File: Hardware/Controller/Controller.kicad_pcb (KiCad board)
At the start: 2 copper layers, 40 parts, among them J2 TagConnect_SWD, Q1 Q_NMOS_GSD, Q3 Q_Dual_NMOS_S1G1S2G2D2D2D1D1, SW1 SW_Push, U1 W25Q64JVXGIQ, U2 AMS1117-3.3, U3 RP2040, U5 LTC4020, Y1 Crystal

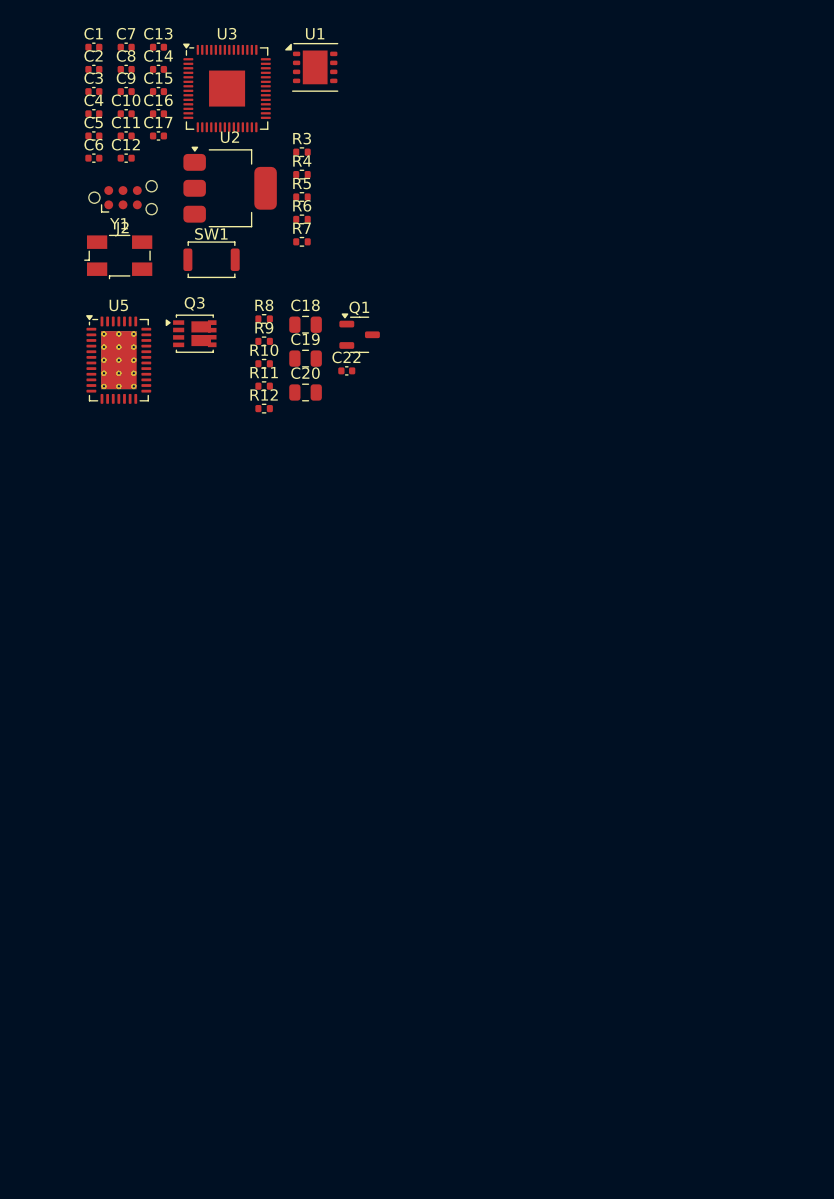
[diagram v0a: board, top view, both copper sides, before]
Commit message: User interface and Controller done
yes
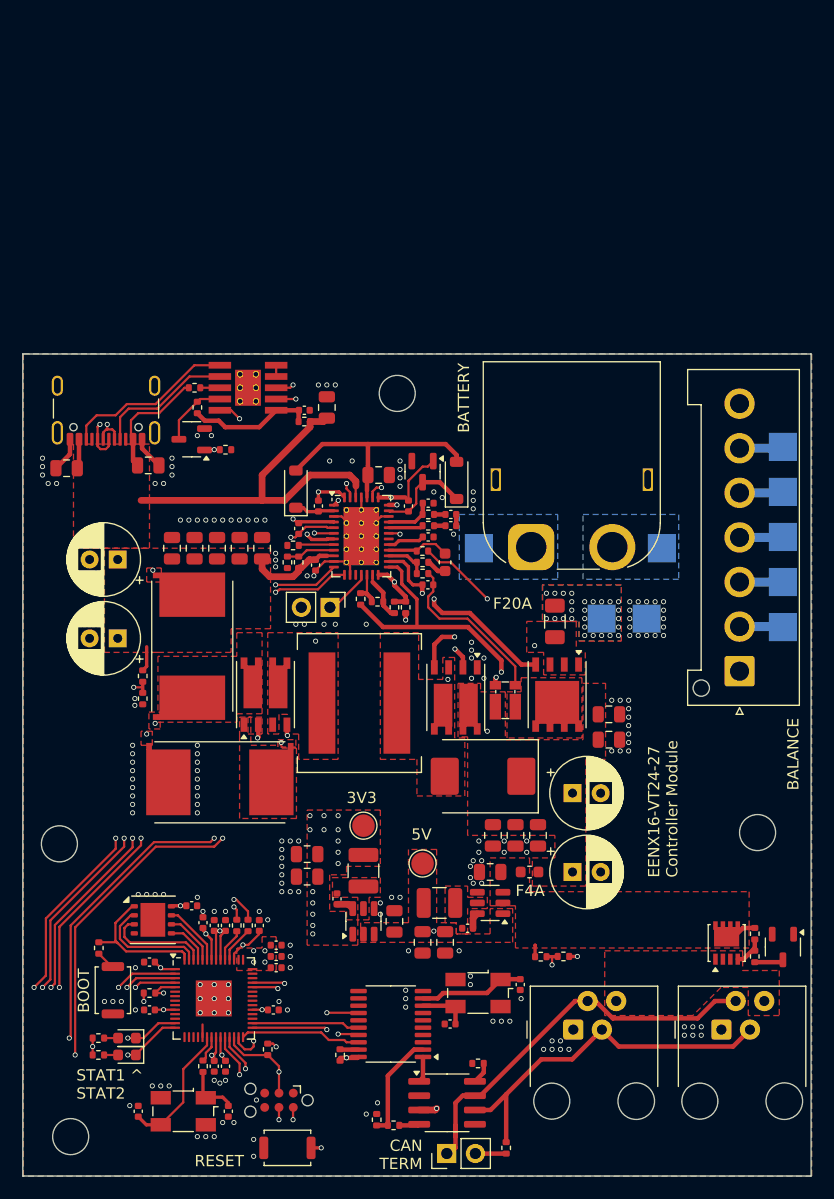
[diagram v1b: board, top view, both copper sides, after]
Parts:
- removed C1, C22, C3, C6: 1u, Capacitor_SMD:C_0402_1005Metric
- removed C10, C11, C12, C13, C14, C15, C16, C17, C2, C7, C8, C9: 100n, Capacitor_SMD:C_0402_1005Metric
- removed C18, C19, C20: 10u, Capacitor_SMD:C_0805_2012Metric
- removed C4, C5: 10p, Capacitor_SMD:C_0402_1005Metric
- removed J2: TagConnect_SWD, Connector:Tag-Connect_TC2030-IDC-NL_2x03_P1.27mm_Vertical
- removed Q1: Q_NMOS_GSD, Package_TO_SOT_SMD:SOT-23-3
- removed Q3: Q_Dual_NMOS_S1G1S2G2D2D2D1D1, Package_SO:Vishay_PowerPAK_1212-8_Dual
- removed R10, R11, R12, R6, R9: 10k, Resistor_SMD:R_0402_1005Metric
- removed R3, R7, R8: 1k, Resistor_SMD:R_0402_1005Metric
- removed R4, R5: 27, Resistor_SMD:R_0402_1005Metric
- removed SW1: SW_Push, Button_Switch_SMD:SW_Push_SPST_NO_Alps_SKRK
- removed U1: W25Q64JVXGIQ, Package_SON:WSON-8-1EP_4x4mm_P0.8mm_EP2.2x3mm
- removed U2: AMS1117-3.3, Package_TO_SOT_SMD:SOT-223-3_TabPin2
- removed U3: RP2040, Package_DFN_QFN:QFN-56-1EP_7x7mm_P0.4mm_EP3.2x3.2mm
- removed U5: LTC4020, Package_DFN_QFN:QFN-38-1EP_5x7mm_P0.5mm_EP3.15x5.15mm_ThermalVias
- removed Y1: Crystal, Crystal:Crystal_SMD_Abracon_ABM3B-4Pin_5.0x3.2mm
- added C201: 100n, Capacitor_SMD:C_0402_1005Metric, F.Cu at (117.0, 129.8)
- added C202: 100n, Capacitor_SMD:C_0402_1005Metric, F.Cu at (117.2, 126.0)
- added C203: 100n, Capacitor_SMD:C_0402_1005Metric, F.Cu at (117.2, 124.0)
- added C204: 100n, Capacitor_SMD:C_0402_1005Metric, F.Cu at (117.2, 125.0)
- added C205: 100n, Capacitor_SMD:C_0402_1005Metric, F.Cu at (112.8, 122.2)
- added C206: 100n, Capacitor_SMD:C_0402_1005Metric, F.Cu at (111.8, 122.2)
- added C207: 100n, Capacitor_SMD:C_0402_1005Metric, F.Cu at (106.0, 125.5)
- added C208: 100n, Capacitor_SMD:C_0402_1005Metric, F.Cu at (106.0, 129.8)
- added C209: 100n, Capacitor_SMD:C_0402_1005Metric, F.Cu at (111.8, 134.8)
- added C210: 1u, Capacitor_SMD:C_0402_1005Metric, F.Cu at (115.8, 122.2)
- added C211: 100n, Capacitor_SMD:C_0402_1005Metric, F.Cu at (110.8, 122.0)
- added C212: 100n, Capacitor_SMD:C_0402_1005Metric, F.Cu at (112.8, 134.8)
- added C213: 100n, Capacitor_SMD:C_0402_1005Metric, F.Cu at (109.8, 120.5)
- added C214: 10p, Capacitor_SMD:C_0402_1005Metric, F.Cu at (105.0, 138.8)
- added C215: 10p, Capacitor_SMD:C_0402_1005Metric, F.Cu at (113.0, 138.8)
- added C301: 10u, Capacitor_SMD:C_0805_2012Metric, F.Cu at (105.9, 81.4)
- added C302: 10u, Capacitor_SMD:C_0805_2012Metric, F.Cu at (98.6, 81.6)
- added C303: 10u, Capacitor_SMD:C_0805_2012Metric, F.Cu at (121.8, 76.2)
- added C304: 1u, Capacitor_SMD:C_0402_1005Metric, F.Cu at (119.8, 76.5)
- added C401: 100n, Capacitor_SMD:C_0402_1005Metric, F.Cu at (122.7, 119.9)
- added C402: 56u, Capacitor_THT:CP_Radial_D6.3mm_P2.50mm, F.Cu at (103.2, 89.8)
- added C403: 56u, Capacitor_THT:CP_Radial_D6.3mm_P2.50mm, F.Cu at (103.2, 96.8)
- added C404: 10u, Capacitor_SMD:C_0805_2012Metric, F.Cu at (112.0, 88.8)
- added C405: 10u, Capacitor_SMD:C_0805_2012Metric, F.Cu at (114.0, 88.8)
- added C406: 10u, Capacitor_SMD:C_0805_2012Metric, F.Cu at (110.0, 88.8)
- added C407: 10u, Capacitor_SMD:C_0805_2012Metric, F.Cu at (108.0, 88.8)
- added C408: 10u, Capacitor_SMD:C_0805_2012Metric, F.Cu at (116.0, 88.8)
- added C409: 10u, Capacitor_SMD:C_0805_2012Metric, F.Cu at (140.5, 114.2)
- added C410: 10u, Capacitor_SMD:C_0805_2012Metric, F.Cu at (138.5, 114.2)
- added C411: 10u, Capacitor_SMD:C_0805_2012Metric, F.Cu at (136.5, 114.2)
- added C412: 10u, Capacitor_SMD:C_0805_2012Metric, F.Cu at (146.8, 105.8)
- added C413: 10u, Capacitor_SMD:C_0805_2012Metric, F.Cu at (146.8, 103.5)
- added C414: 56u, Capacitor_THT:CP_Radial_D6.3mm_P2.50mm, F.Cu at (143.6, 110.5)
- added C415: 56u, Capacitor_THT:CP_Radial_D6.3mm_P2.50mm, F.Cu at (143.6, 117.5)
- added C416: 10u, Capacitor_SMD:C_0805_2012Metric, F.Cu at (127.8, 121.9)
- added C417: 22u, Capacitor_SMD:C_0805_2012Metric, F.Cu at (120.0, 115.9)
- added C418: 22u, Capacitor_SMD:C_0805_2012Metric, F.Cu at (120.0, 117.9)
- added C419: 100n, Capacitor_SMD:C_0402_1005Metric, F.Cu at (134.2, 122.5)
- added C420: 10u, Capacitor_SMD:C_0805_2012Metric, F.Cu at (136.2, 117.5)
- added C421: 22u, Capacitor_SMD:C_0805_2012Metric, F.Cu at (132.2, 123.8)
- added C422: 22u, Capacitor_SMD:C_0805_2012Metric, F.Cu at (130.2, 123.8)
- added C423: 1u, Capacitor_SMD:C_0402_1005Metric, F.Cu at (121.0, 85.0)
- added C424: 1u, Capacitor_SMD:C_0402_1005Metric, F.Cu at (129.0, 85.0)
- added C425: 2u2, Capacitor_SMD:C_0603_1608Metric, F.Cu at (132.2, 90.0)
- added C426: 1n, Capacitor_SMD:C_0402_1005Metric, F.Cu at (130.7, 92.0)
- added C427: 10u, Capacitor_SMD:C_0805_2012Metric, F.Cu at (126.3, 82.2)
- added C428: 10n, Capacitor_SMD:C_0402_1005Metric, F.Cu at (132.8, 86.8)
- added C429: 680p, Capacitor_SMD:C_0402_1005Metric, F.Cu at (132.8, 85.8)
- added C430: 68p, Capacitor_SMD:C_0402_1005Metric, F.Cu at (130.8, 84.8)
- added C431: 100p, Capacitor_SMD:C_0402_1005Metric, F.Cu at (130.8, 87.8)
- added C432: 100n, Capacitor_SMD:C_0402_1005Metric, F.Cu at (120.8, 90.2)
- added C433: 33n, Capacitor_SMD:C_0402_1005Metric, F.Cu at (119.2, 87.0)
- added C501: 10p, Capacitor_SMD:C_0402_1005Metric, F.Cu at (132.7, 131.0)
- added C502: 10p, Capacitor_SMD:C_0402_1005Metric, F.Cu at (138.9, 127.5)
- added D401: MBRS360, Diode_SMD:D_SMC, F.Cu at (135.6, 109.0)
- added D402: BZX84C6V2L, Package_TO_SOT_SMD:SOT-23, F.Cu at (130.2, 82.0)
- added D403: SBR0560S1, Diode_SMD:D_SOD-123, F.Cu at (119.0, 83.5)
- added D404: SBR0560S1, Diode_SMD:D_SOD-123, F.Cu at (133.3, 82.7)
- added D405: LED-GREEN, LED_SMD:LED_0603_1608Metric, F.Cu at (104.0, 132.2)
- added D406: LED-GREEN, LED_SMD:LED_0603_1608Metric, F.Cu at (104.0, 133.8)
- added F401: 5A, Fuse:Fuse_0603_1608Metric, F.Cu at (139.8, 117.5)
- added F402: 20A, Fuse:Fuse_1206_3216Metric, F.Cu at (142.0, 95.2)
- added H101: MountingHole, MountingHole:MountingHole_3.2mm_M3, F.Cu at (160.0, 114.0)
- added H102: MountingHole, MountingHole:MountingHole_3.2mm_M3, F.Cu at (128.0, 75.0)
- added H103: MountingHole, MountingHole:MountingHole_3.2mm_M3, F.Cu at (98.0, 115.0)
- added H104: MountingHole, MountingHole:MountingHole_3.2mm_M3, F.Cu at (99.0, 141.0)
- added J201: TagConnect_SWD, Connector:Tag-Connect_TC2030-IDC-NL_2x03_P1.27mm_Vertical, F.Cu at (117.5, 137.8)
- added J301: USB_C_Receptacle_USB2.0_16P, Connector_USB:USB_C_Receptacle_GCT_USB4105-xx-A_16P_TopMnt_Horizontal, F.Cu at (102.1, 75.4)
- added J401: XT60, Connector_AMASS:AMASS_XT60PW-M_1x02_P7.20mm_Horizontal, F.Cu at (139.9, 88.7)
- added J402: Conn_balance, Connector_JST:JST_VH_B7P-VH-FB-B_1x07_P3.96mm_Vertical, F.Cu at (158.4, 99.7)
- added J403: Conn_NTC, Connector_PinHeader_2.54mm:PinHeader_1x02_P2.54mm_Vertical, F.Cu at (122.0, 94.0)
- added J501: RJ9, Connector_RJ:RJ9_Evercom_5301-440xxx_Horizontal, F.Cu at (143.6, 131.5)
- added J502: RJ9, Connector_RJ:RJ9_Evercom_5301-440xxx_Horizontal, F.Cu at (156.8, 131.5)
- added JP501: Jumper_termination, Connector_PinHeader_2.54mm:PinHeader_1x02_P2.54mm_Vertical, F.Cu at (132.4, 142.5)
- added L401: 4u7, Inductor_SMD:L_1210_3225Metric, F.Cu at (125.0, 117.4)
- added L402: XAL1010-153MED, Inductor_SMD:L_Coilcraft_XAL1010-XXX, F.Cu at (124.6, 102.5)
- added L403: 4u7, Inductor_SMD:L_1210_3225Metric, F.Cu at (131.8, 120.2)
- added Q301: Q_NMOS_GSD, Package_TO_SOT_SMD:SOT-23-3, F.Cu at (109.8, 79.1)
- added Q401: Si7252DP, Package_SO:PowerPAK_SO-8_Dual, F.Cu at (116.3, 101.8)
- added Q402: Si7252DP, Package_SO:PowerPAK_SO-8_Dual, F.Cu at (133.2, 102.0)
- added Q403: Si7461DP, Package_SO:PowerPAK_SO-8_Single, F.Cu at (142.2, 101.8)
- added Q501: Si7461DP, Package_SO:Vishay_PowerPAK_1212-8_Single, F.Cu at (157.2, 123.8)
- added Q502: Q_NMOS_GSD, Package_TO_SOT_SMD:SOT-23-3, F.Cu at (162.2, 124.2)
- added R201: 10k, Resistor_SMD:R_0402_1005Metric, F.Cu at (116.5, 133.2)
- added R202: 1k, Resistor_SMD:R_0402_1005Metric, F.Cu at (101.5, 124.2)
- added R203: 27, Resistor_SMD:R_0402_1005Metric, F.Cu at (113.8, 122.2)
- added R204: 27, Resistor_SMD:R_0402_1005Metric, F.Cu at (114.8, 122.2)
- added R205: 1k, Resistor_SMD:R_0402_1005Metric, F.Cu at (110.8, 134.8)
- added R301: 1k, Resistor_SMD:R_0402_1005Metric, F.Cu at (119.8, 77.5)
- added R302: 10k, Resistor_SMD:R_0402_1005Metric, F.Cu at (110.0, 74.5)
- added R303: 10k, Resistor_SMD:R_0402_1005Metric, F.Cu at (106.0, 128.2)
- added R304: 10k, Resistor_SMD:R_0402_1005Metric, F.Cu at (110.2, 76.2)
- added R305: 10k, Resistor_SMD:R_0402_1005Metric, F.Cu at (112.8, 80.0)
- added R401: 8m, personal:R_Shunt_Vishay_WSR2_WSR3_KelvinConnection_4pins, F.Cu at (109.5, 97.5)
- added R402: 8m, personal:R_Shunt_Vishay_WSR2_WSR3_KelvinConnection_4pins, F.Cu at (112.2, 109.2)
- added R403: 100, Resistor_SMD:R_0402_1005Metric, F.Cu at (130.2, 89.0)
- added R404: 105k, Resistor_SMD:R_0402_1005Metric, F.Cu at (119.2, 90.0)
- added R405: 215k, Resistor_SMD:R_0402_1005Metric, F.Cu at (128.8, 94.0)
- added R406: 215k, Resistor_SMD:R_0402_1005Metric, F.Cu at (124.8, 93.2)
- added R407: 2m, Resistor_SMD:R_Shunt_Vishay_WSKW0612, F.Cu at (137.6, 102.2)
- added R408: 100, Resistor_SMD:R_0402_1005Metric, F.Cu at (130.2, 91.0)
- added R409: 4R7, Resistor_SMD:R_0402_1005Metric, F.Cu at (130.2, 90.0)
- added R410: 10k, Resistor_SMD:R_0402_1005Metric, F.Cu at (118.2, 90.0)
- added R411: 24k9, Resistor_SMD:R_0402_1005Metric, F.Cu at (127.8, 94.0)
- added R412: 24k9, Resistor_SMD:R_0402_1005Metric, F.Cu at (126.2, 93.5)
- added R413: 100k, Resistor_SMD:R_0402_1005Metric, F.Cu at (118.8, 88.5)
- added R414: 56k, Resistor_SMD:R_0402_1005Metric, F.Cu at (130.8, 86.8)
- added R415: 47k, Resistor_SMD:R_0402_1005Metric, F.Cu at (130.8, 85.8)
- added R416: 1k, Resistor_SMD:R_0402_1005Metric, F.Cu at (101.5, 132.2)
- added R417: 1k, Resistor_SMD:R_0402_1005Metric, F.Cu at (101.5, 133.8)
- added R418: 1k, Resistor_SMD:R_0402_1005Metric, F.Cu at (105.4, 102.1)
- added R419: 1k, Resistor_SMD:R_0402_1005Metric, F.Cu at (142.8, 125.0)
- added R420: 10k, Resistor_SMD:R_0402_1005Metric, F.Cu at (140.8, 125.0)
- added R421: 10k, Resistor_SMD:R_0402_1005Metric, F.Cu at (105.4, 100.1)
- added R501: 10k, Resistor_SMD:R_0402_1005Metric, F.Cu at (159.8, 123.0)
- added R502: 5k1, Resistor_SMD:R_0402_1005Metric, F.Cu at (159.8, 125.0)
- added R503: 120, Resistor_SMD:R_0402_1005Metric, F.Cu at (137.7, 142.0)
- added R504: 5k1, Resistor_SMD:R_0402_1005Metric, F.Cu at (127.7, 140.0)
- added R505: 10k, Resistor_SMD:R_0402_1005Metric, F.Cu at (126.2, 139.5)
- added R506: 10k, Resistor_SMD:R_0402_1005Metric, F.Cu at (135.2, 134.5)
- added R507: 10k, Resistor_SMD:R_0402_1005Metric, F.Cu at (122.9, 133.8)
- added SW201: SW_Push, Button_Switch_SMD:SW_Push_SPST_NO_Alps_SKRK, F.Cu at (118.2, 142.0)
- added SW202: SW_Push, Button_Switch_SMD:SW_Push_SPST_NO_Alps_SKRK, F.Cu at (102.8, 128.0)
- added TP401: TP3V3, TestPoint:TestPoint_Pad_D2.0mm, F.Cu at (125.0, 113.4)
- added TP402: TP5V, TestPoint:TestPoint_Pad_D2.0mm, F.Cu at (130.2, 116.8)
- added TP403: BAT_S5, TestPoint:TestPoint_Pad_2.5x2.5mm, B.Cu at (162.2, 79.8)
- added TP404: BAT_PROT+, TestPoint:TestPoint_Pad_2.5x2.5mm, B.Cu at (146.2, 95.0)
- added TP405: BAT_UNPROT+, TestPoint:TestPoint_Pad_2.5x2.5mm, B.Cu at (151.5, 88.8)
- added TP406: BAT_S4, TestPoint:TestPoint_Pad_2.5x2.5mm, B.Cu at (162.2, 83.8)
- added TP407: BAT_PROT-, TestPoint:TestPoint_Pad_2.5x2.5mm, B.Cu at (150.2, 95.0)
- added TP408: BAT_UNPROT-, TestPoint:TestPoint_Pad_2.5x2.5mm, B.Cu at (135.2, 88.8)
- added TP409: BAT_S3, TestPoint:TestPoint_Pad_2.5x2.5mm, B.Cu at (162.2, 87.8)
- added TP410: BAT_S2, TestPoint:TestPoint_Pad_2.5x2.5mm, B.Cu at (162.2, 91.8)
- added TP411: BAT_S1, TestPoint:TestPoint_Pad_2.5x2.5mm, B.Cu at (162.2, 95.8)
- added U201: W25Q64JVXGIQ, Package_SON:WSON-8-1EP_4x4mm_P0.8mm_EP2.2x3mm, F.Cu at (106.3, 121.8)
- added U202: RP2040, Package_DFN_QFN:QFN-56-1EP_7x7mm_P0.4mm_EP3.2x3.2mm, F.Cu at (111.7, 128.7)
- added U301: CH224K, WCH:ESSOP10, F.Cu at (114.8, 74.5)
- added U401: AP63203WU, Package_TO_SOT_SMD:TSOT-23-6, F.Cu at (125.0, 121.9)
- added U402: AP63205WU, Package_TO_SOT_SMD:TSOT-23-6, F.Cu at (136.2, 120.2)
- added U403: LTC4020, Package_DFN_QFN:QFN-38-1EP_5x7mm_P0.5mm_EP3.15x5.15mm_ThermalVias, F.Cu at (124.8, 87.7)
- added U501: MCP2551-I-SN, Package_SO:SOIC-8_3.9x4.9mm_P1.27mm, F.Cu at (132.4, 138.0)
- added U502: MCP2515-xST, Package_SO:TSSOP-20_4.4x6.5mm_P0.65mm, F.Cu at (127.4, 131.0)
- added Y201: 12M, Crystal:Crystal_SMD_Abracon_ABM3B-4Pin_5.0x3.2mm, F.Cu at (109.0, 138.8)
- added Y501: 8M, Crystal:Crystal_SMD_Abracon_ABM3B-4Pin_5.0x3.2mm, F.Cu at (135.2, 128.2)
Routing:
- net /CFG3: track 0.00 -> 77.2 mm, vias 0 -> 4
- net /CFG2: track 0.00 -> 75.7 mm, vias 0 -> 4
- net /PG: track 0.00 -> 75.5 mm, vias 0 -> 4
- net /~{CFG1}: track 0.00 -> 69.9 mm, vias 0 -> 4
- net /STAT2_OUT: track 0.00 -> 68.2 mm, vias 0 -> 4
- net /STAT1_OUT: track 0.00 -> 66.6 mm, vias 0 -> 4
- net /USB_D+: track 0.00 -> 59.4 mm, vias 0 -> 2
- net /USB_D-: track 0.00 -> 58.8 mm, vias 0 -> 2
- net VBUS: track 0.00 -> 56.7 mm
- net /VBUS_MONITOR: track 0.00 -> 39.5 mm, vias 0 -> 2
- net /CAN_bus/CANH: track 0.00 -> 35.6 mm
- net /CAN_bus/CANL: track 0.00 -> 32.9 mm
- net /Battery/BG1: track 0.00 -> 32.4 mm, vias 0 -> 2
- net /Battery/SW2: track 0.00 -> 29.6 mm, vias 0 -> 2
- net /BATTERY_MONITOR: track 0.00 -> 29.0 mm, vias 0 -> 2
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- added copper zone on F.Cu, net +3V3
- added copper zone on In2.Cu, net +3V3
- added copper zone on F.Cu, net +5V
- added copper zone on F.Cu, net +SYSTEM
- added copper zone on F.Cu, net /Battery/BAT
- added copper zone on F.Cu, net /Battery/BATT_RAW
- added copper zone on F.Cu, net /Battery/SENSBOT
- added copper zone on F.Cu, net /Battery/SENSGND
- added copper zone on F.Cu, net /Battery/SENSTOP
- added copper zone on F.Cu, net /Battery/SENSVin
- added copper zone on F.Cu, net /Battery/SW1
- added copper zone on F.Cu, net /Battery/SW2
- added copper zone on B.Cu, net GND
- added copper zone on F.Cu, net GND
- added copper zone on In1.Cu, net GND
- added copper zone on In2.Cu, net GND
- added copper zone on B.Cu, net Net-(F402-Pad2)
- added copper zone on F.Cu, net Net-(F402-Pad2)
- added copper zone on B.Cu, net Net-(J401-Pin_1)
- added copper zone on B.Cu, net Net-(J401-Pin_2)
- added copper zone on F.Cu, net Net-(J501-Pad4)
- added copper zone on F.Cu, net Net-(Q401A-S)
- added copper zone on F.Cu, net Net-(Q401B-D)
- added copper zone on F.Cu, net Net-(Q403-D)
- added copper zone on F.Cu, net Net-(U401-SW)
- added copper zone on F.Cu, net Net-(U402-SW)
- added copper zone on F.Cu, net VBUS
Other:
- board outline added: 70 x 73 mm
- copper layers 2 -> 4
- board text added: "3V3"
- board text added: "5V"
- board text added: "BALANCE"
- board text added: "BATTERY"
- board text added: "BOOT"
- board text added: "CAN TERM"
- board text added: "EENX16-VT24-27 Controller Module"
- board text added: "F20A"
- board text added: "F4A"
- board text added: "RESET"
- board text added: "STAT1 ^ STAT2"
